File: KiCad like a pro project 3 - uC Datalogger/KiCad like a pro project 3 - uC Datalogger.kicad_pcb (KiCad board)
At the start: 2 copper layers, 53.8 x 34 mm, 30 parts, among them J1 Conn_01x04_Male, J2 Conn_01x09_Male, J3 Conn_01x04_Male, J4 Conn_02x03_Odd_Even, U1 24LC1025, U2 24LC1025, U3 DS1337S+, U4 ATMEGA328P_VQFNVQFN, Y1 32.768 KHz, Y2 16 MHz

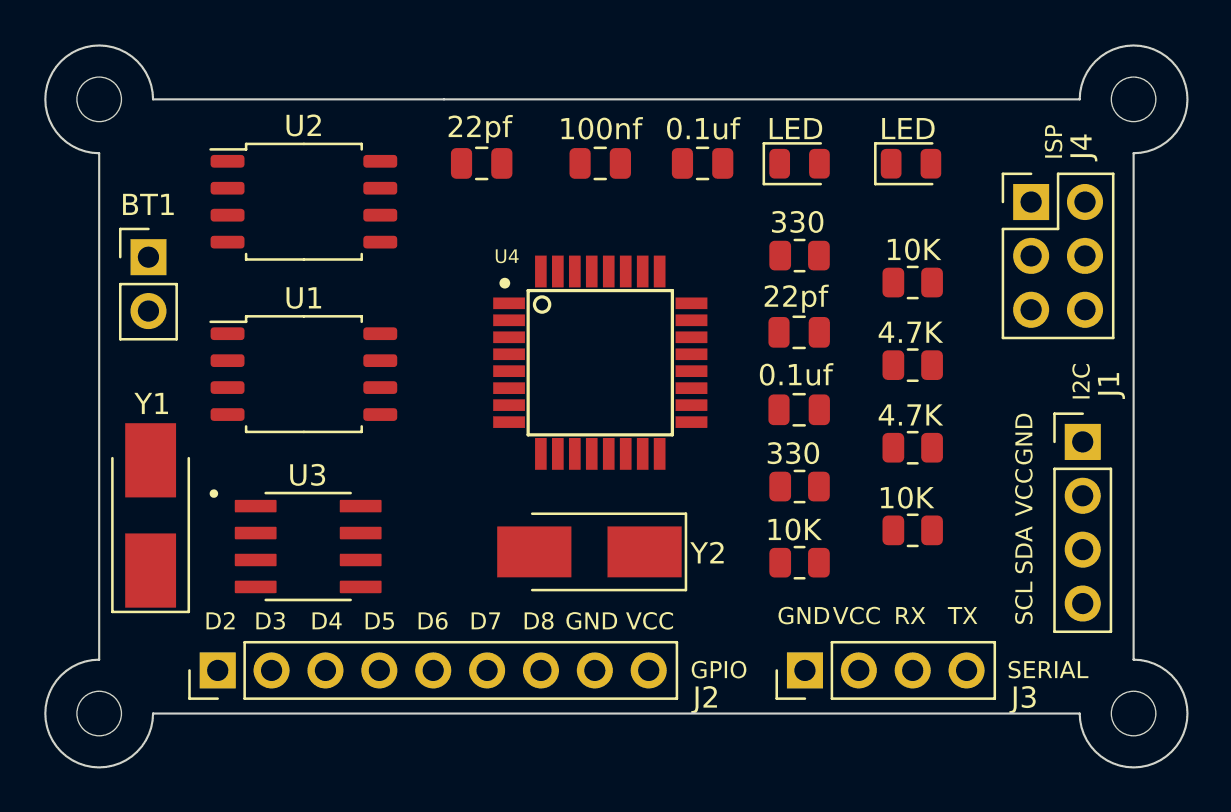
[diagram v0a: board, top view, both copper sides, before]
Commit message: Finished wiring
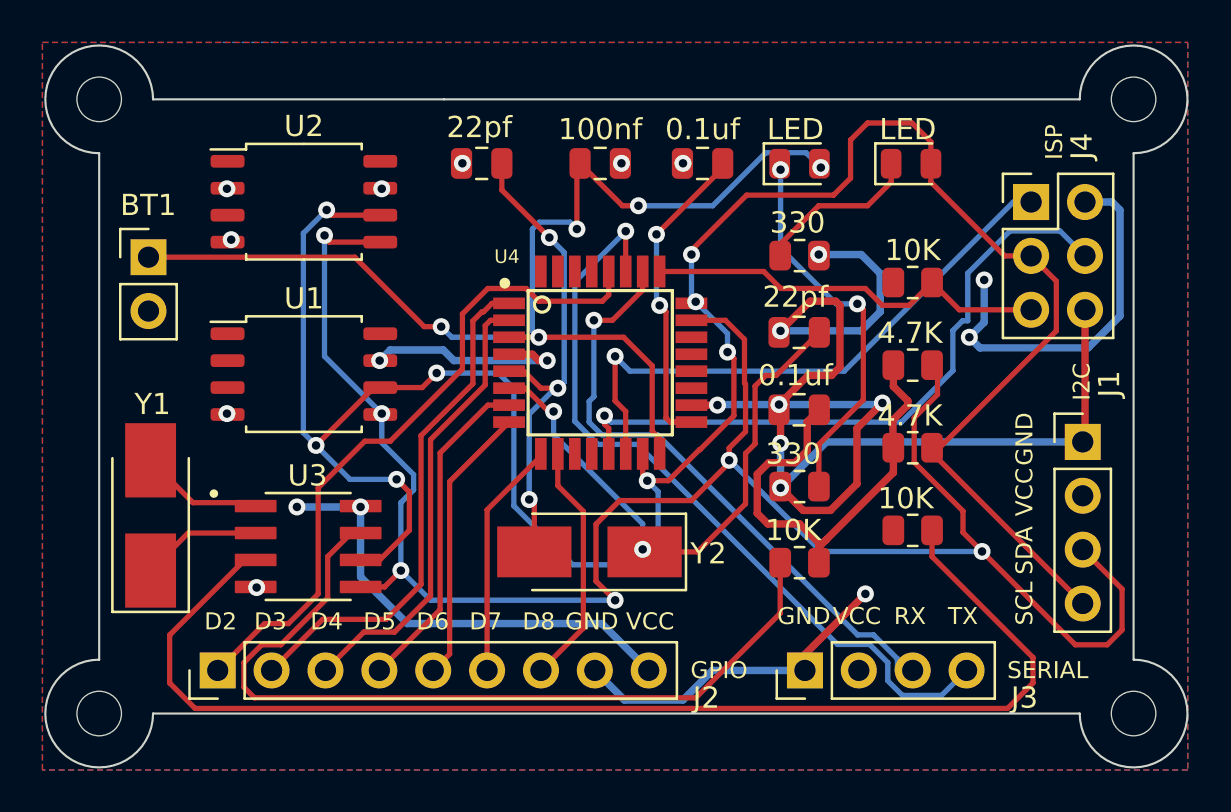
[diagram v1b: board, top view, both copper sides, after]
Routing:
- net /SCL: track 0.00 -> 113.9 mm, vias 0 -> 8
- net /SDA: track 0.00 -> 91.6 mm, vias 0 -> 6
- net GND: track 0.00 -> 89.8 mm, vias 0 -> 18
- net /Vcc: track 0.00 -> 61.3 mm, vias 0 -> 4
- net Net-(R2-Pad2): track 0.00 -> 58.6 mm
- net Net-(BT1-Pad1): track 0.00 -> 55.8 mm, vias 0 -> 5
- net Net-(R4-Pad2): track 0.00 -> 39.9 mm
- net /TX: track 0.00 -> 36.7 mm, vias 0 -> 1
- net /D2: track 0.00 -> 31.8 mm
- net /MOSI: track 0.00 -> 31.3 mm, vias 0 -> 1
- net /RX: track 0.00 -> 29.1 mm, vias 0 -> 1
- net /MISO: track 0.00 -> 28.0 mm, vias 0 -> 1
- net Net-(U4-Pad6): track 0.00 -> 26.3 mm, vias 0 -> 2
- net /D3: track 0.00 -> 24.2 mm
- net Net-(U4-Pad5): track 0.00 -> 23.6 mm, vias 0 -> 3
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- added copper zone on F.Cu, net /Vcc
- added copper zone on B.Cu, net GND
